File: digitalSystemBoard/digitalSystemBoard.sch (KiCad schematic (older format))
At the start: 39 parts, among them J1 Barrel_Jack, J10 Conn_02x08_Odd_Even, J11 Conn_02x03_Odd_Even, J13 Conn_02x03_Odd_Even, J3 7_LED_IN_2, J4 7_LED_IN_1, J5 INPUT_HEADER, J6 SN7447, J7 SN7447, J9 Conn_02x08_Odd_Even, Q1 MJD122T4G, SW1 SW_SPDT, SW2 ButtonFirst, SW3 ButtonFirst, U1 LM317, U15 KCSA02-105, U16 KCSA02-105, U2 Potentiometer, U20 74HC04

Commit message: Hot fix libs. Update schematic
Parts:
- removed V0, V1, V2, V3, V4: POWER_VIAS, digitalSystemBoard:POWER_VIA, symbol digitalSystemBoard-rescue:POWER_VIAS
- SW2, SW3: symbol digitalSystemBoard-rescue:ButtonFirst-project -> digitalSystemBoard:ButtonFirst
- U1: symbol digitalSystemBoard-rescue:LM317-digitalSystemBoard -> digitalSystemBoard:LM317
- U2: symbol digitalSystemBoard-rescue:Potentiometer-digitalSystemBoard -> digitalSystemBoard:Potentiometer
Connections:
- net labels removed: VIA_0, VIA_1
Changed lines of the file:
@@
 $EndComp
 $Comp
-L digitalSystemBoard-rescue:ButtonFirst-project SW2
+L digitalSystemBoard:ButtonFirst SW2
 U 1 1 5F8C8A55
 P 1742 5100
@@
 $EndComp
 $Comp
-L digitalSystemBoard-rescue:ButtonFirst-project SW3
+L digitalSystemBoard:ButtonFirst SW3
 U 1 1 5F8DA262
 P 3048 5068
@@
 	2016 2108 2556 2108
 $Comp
-L digitalSystemBoard-rescue:Potentiometer-digitalSystemBoard U2
+L digitalSystemBoard:Potentiometer U2
 U 1 1 5F873747
 P 2556 1632
@@
 	1810 1266 1810 2108
 $Comp
-L digitalSystemBoard-rescue:LM317-digitalSystemBoard U1
+L digitalSystemBoard:LM317 U1
 U 1 1 5F871BB7
 P 2556 1082
@@
 Wire Wire Line
 	3922 2932 3972 2932
-$Comp
-L digitalSystemBoard-rescue:POWER_VIAS V0
-U 1 1 5F9A9094
-P 988 2716
-F 0 "V0" V 1092 2538 50  0000 R CNN
-F 1 "POWER_VIAS" V 1001 2538 50  0000 R CNN
-F 2 "digitalSystemBoard:POWER_VIA" H 988 2716 50  0001 C CNN
-F 3 "" H 988 2716 50  0001 C CNN
-	1    988  2716
-	0    -1   -1   0
-$EndComp
-Text Label 988  2366 0    50   ~ 0
-VIA_0
-Text Label 3924 806  0    50   ~ 0
-VIA_0
-$Comp
-L digitalSystemBoard-rescue:POWER_VIAS V1
-U 1 1 5F9C57FC
-P 1758 2792
-F 0 "V1" V 1862 2614 50  0000 R CNN
-F 1 "POWER_VIAS" V 1771 2614 50  0000 R CNN
-F 2 "digitalSystemBoard:POWER_VIA" H 1758 2792 50  0001 C CNN
-F 3 "" H 1758 2792 50  0001 C CNN
-	1    1758 2792
-	0    -1   -1   0
-$EndComp
-$Comp
-L digitalSystemBoard-rescue:POWER_VIAS V2
-U 1 1 5F9C895C
-P 2542 2764
-F 0 "V2" V 2646 2586 50  0000 R CNN
-F 1 "POWER_VIAS" V 2555 2586 50  0000 R CNN
-F 2 "digitalSystemBoard:POWER_VIA" H 2542 2764 50  0001 C CNN
-F 3 "" H 2542 2764 50  0001 C CNN
-	1    2542 2764
-	0    -1   -1   0
-$EndComp
-Text Label 1758 2442 0    50   ~ 0
-VIA_0
-Text Label 2542 2414 0    50   ~ 0
-VIA_0
-$Comp
-L digitalSystemBoard-rescue:POWER_VIAS V3
-U 1 1 5FA14C14
-P 802 1888
-F 0 "V3" V 906 1710 50  0000 R CNN
-F 1 "POWER_VIAS" V 790 2122 50  0000 R CNN
-F 2 "digitalSystemBoard:POWER_VIA" H 802 1888 50  0001 C CNN
-F 3 "" H 802 1888 50  0001 C CNN
-	1    802  1888
-	0    -1   -1   0
-$EndComp
-Text Label 3032 1680 0    50   ~ 0
-VIA_1
-Text Label 802  1538 0    50   ~ 0
-VIA_1
-$Comp
-L digitalSystemBoard-rescue:POWER_VIAS V4
-U 1 1 5FA1E10B
-P 1232 1874
-F 0 "V4" V 1336 1696 50  0000 R CNN
-F 1 "POWER_VIAS" V 1208 2102 50  0000 R CNN
-F 2 "digitalSystemBoard:POWER_VIA" H 1232 1874 50  0001 C CNN
-F 3 "" H 1232 1874 50  0001 C CNN
-	1    1232 1874
-	0    -1   -1   0
-$EndComp
-Text Label 1232 1524 0    50   ~ 0
-VIA_1
 $EndSCHEMATC

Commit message: Update new schematic.
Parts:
- removed H0, H1, H2, H3: MountingHole, MountingHole:MountingHole_3.2mm_M3, symbol Mechanical:MountingHole
- removed J10, J9: Conn_02x08_Odd_Even, Connector_PinHeader_2.54mm:PinHeader_2x08_P2.54mm_Vertical_SMD, symbol Connector_Generic:Conn_02x08_Odd_Even
- removed J11, J13: Conn_02x03_Odd_Even, Connector_PinHeader_2.54mm:PinHeader_2x03_P2.54mm_Vertical_SMD, symbol Connector_Generic:Conn_02x03_Odd_Even
- removed J3: 7_LED_IN_2, Connector_PinHeader_2.54mm:PinHeader_2x07_P2.54mm_Vertical_SMD, symbol Connector_Generic:Conn_02x07_Odd_Even
- removed J4: 7_LED_IN_1, Connector_PinHeader_2.54mm:PinHeader_2x07_P2.54mm_Vertical_SMD, symbol Connector_Generic:Conn_02x07_Odd_Even
- removed J5: INPUT_HEADER, Connector_PinHeader_2.54mm:PinHeader_2x12_P2.54mm_Vertical_SMD, symbol Connector_Generic:Conn_02x12_Odd_Even
- removed J6, J7: SN7447, digitalSystemBoard:SN7447, symbol Connector_Generic:Conn_02x08_Odd_Even
- removed Q1: MJD122T4G, digitalSystemBoard:MJD122T4G, symbol Device:Q_NPN_BCE
- removed R4, R5: 10K, Resistor_SMD:R_0603_1608Metric, symbol Device:R
- removed SW2, SW3: ButtonFirst, digitalSystemBoard:Button, symbol digitalSystemBoard:ButtonFirst
- removed U15, U16: KCSA02-105, Display_7Segment:7SegmentLED_LTS6760_LTS6780, symbol Display_Character:KCSA02-105
- removed U2: Potentiometer, digitalSystemBoard:TRIM_3296W-1-501, symbol digitalSystemBoard:Potentiometer
- removed U20: 74HC04, Package_SO:SOIC-14_3.9x8.7mm_P1.27mm, symbol 74xx:74HC04
- added J2, J3: Conn_02x02_Odd_Even, symbol Connector_Generic:Conn_02x02_Odd_Even
- added Q1: MJD122T4G, symbol digitalSystemBoard:MJD122T4G
- added TRIM1: Potentiometer, symbol digitalSystemBoard:Potentiometer
- C1, C3, C4: footprint Capacitor_SMD:C_0603_1608Metric -> (none)
- C2: value 100uF_C -> 100uF; footprint Capacitor_SMD:CP_Elec_5x5.8 -> (none)
- D1: footprint LED_SMD:LED_0805_2012Metric -> (none)
- F1: footprint digitalSystemBoard:Fuse -> (none)
- J1: footprint footprints:BARREL_JACK -> (none)
- R1, R3: footprint Resistor_SMD:R_0603_1608Metric -> (none)
- R2: value 0.22Ohm_5W -> 0.22_5W; footprint digitalSystemBoard:5W_0.22R -> (none)
- SW1: footprint digitalSystemBoard:SS-12D11 -> (none)
- U1: footprint digitalSystemBoard:TO228P991X255-3N -> (none)
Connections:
- net labels added: ADJ_CLOCK, BCD_A_0, BCD_A_1, BCD_B_0, BCD_B_1, BCD_C_0, BCD_C_1, BCD_D_0, BCD_D_1, CHANGE_CLK_SRC, DOWN_CLOCK, LED1, LED2, LED3, LED4, LED5, LED6, LED7, LED8, UP_CLOCK, VCC5V
- net labels removed: A1, A2, A_J, A_K, A_X, A_Y, B1, B2, BI_RBO, B_J, B_K, B_X, B_Y, C1, C2, CLK_OUT, C_J, C_K, C_X, C_Y, D1, D2, D_J, D_K, D_X, D_Y, E_J, E_K, E_X, E_Y, F_J, F_K, F_X, F_Y, G_J, G_K, G_X, G_Y, IB1, IB2, LT, O1, O10, O2, O3, O4, O5, O6, O7, O8, O9, OA1, OA2, OB1, OB2, OC1, OC2, OD1, OD2, OLED1, OLED2, OLED3, OLED4, OLED5, OLED6, OLED7, OLED8, RBI, TLED1, TLED2, TLED3, TLED4, TLED5, TLED6, TLED7, TLED8, VCC, VIN
- wire segments 96 -> 35
- no-connect marks 7 -> 2
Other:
- note removed: "CLOCK_BLOCK\n"
- note removed: "INPUT_BLOCK"
- note removed: "OUTPUT_BLOCK\n"
- note removed: "SOURCE_BLOCK\n"

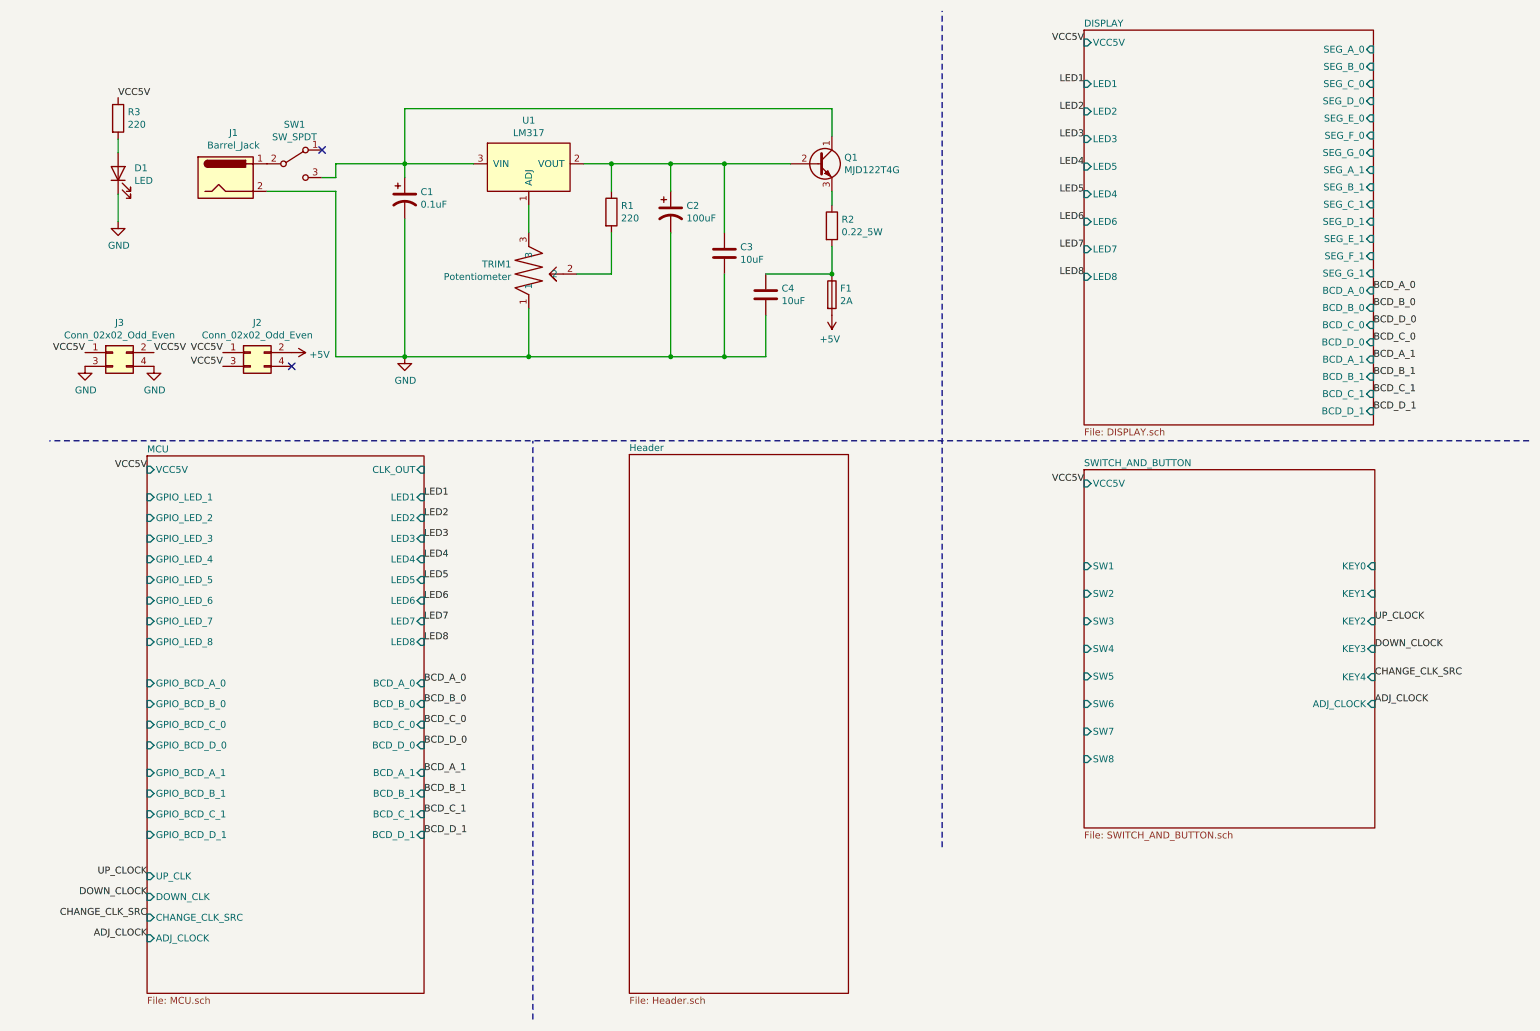
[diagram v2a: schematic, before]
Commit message: Change grid size to 10mils and wire components in power supply and display sheet
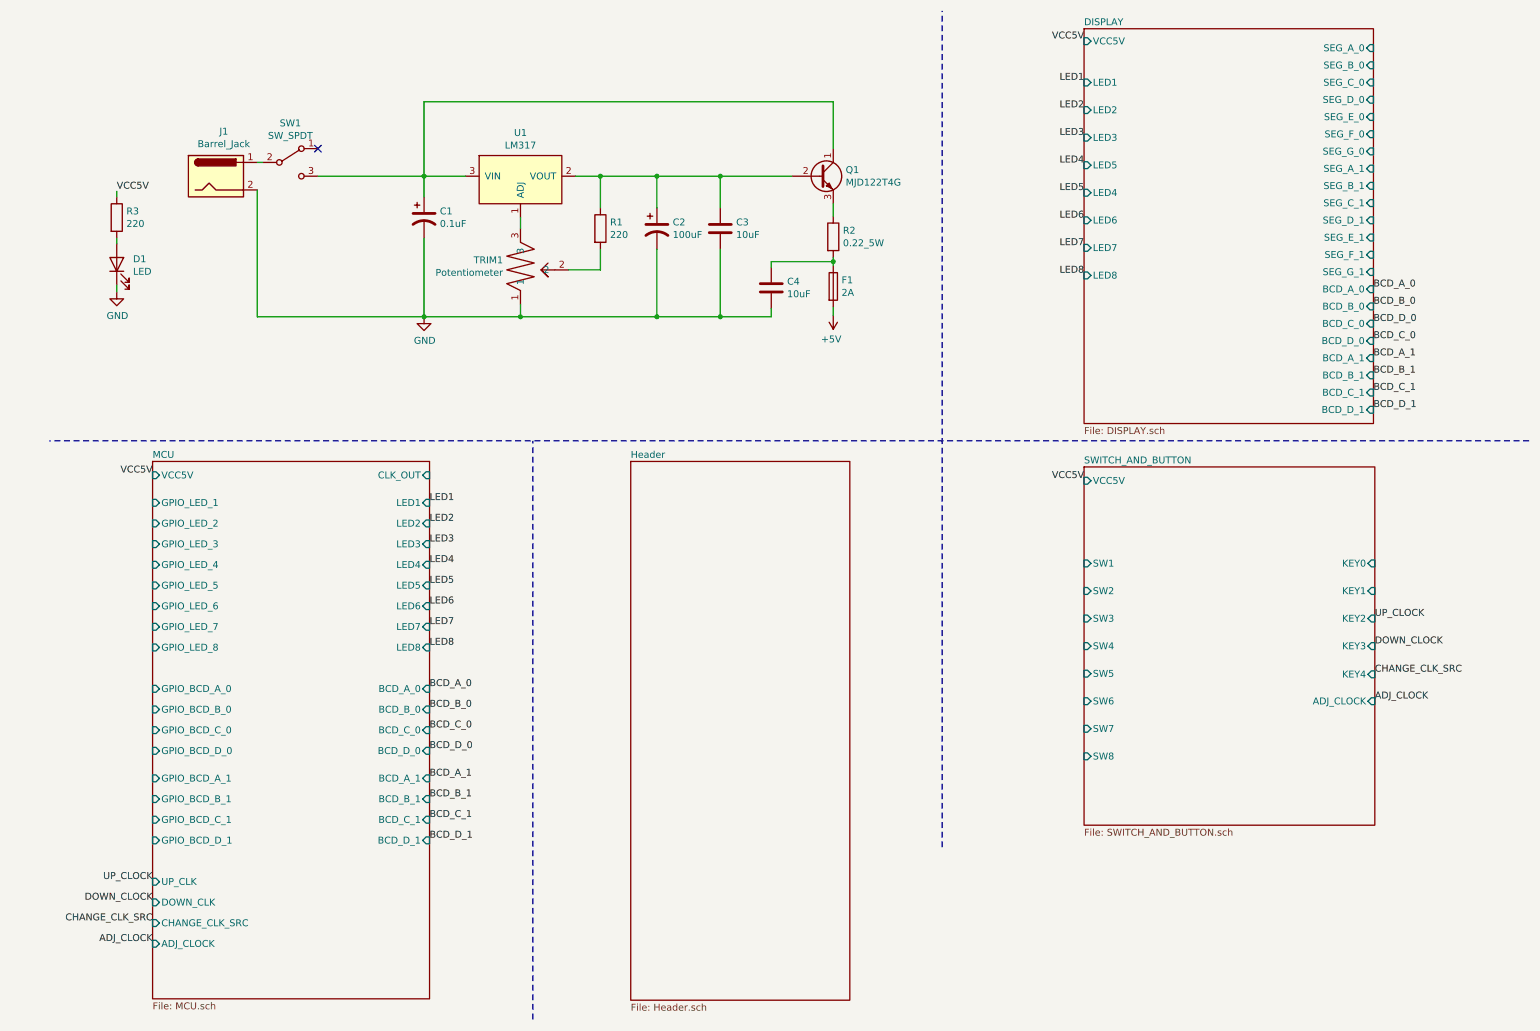
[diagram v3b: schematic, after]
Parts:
- removed J2, J3: Conn_02x02_Odd_Even, symbol Connector_Generic:Conn_02x02_Odd_Even
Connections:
- no-connect marks 2 -> 1
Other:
- moved on the sheet: C1, C2, C3, C4, D1, F1, J1, Q1, R1, R2, R3, SW1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
